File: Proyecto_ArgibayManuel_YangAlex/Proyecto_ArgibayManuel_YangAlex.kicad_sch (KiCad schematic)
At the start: 27 parts, among them J2 Conn_01x04, J3 Conn_01x06, J4 Conn_01x05, SW1 SW_Push, SW2 SW_Push, SW3 SW_Push, SW4 SW_Push, U1 PIC18F258-I_SO, U2 LT1716IS5TRMPBF, U3 LT1716IS5TRMPBF, U7 HDC2010YPAR, U8 TXS0108EPW, Y1 Crystal

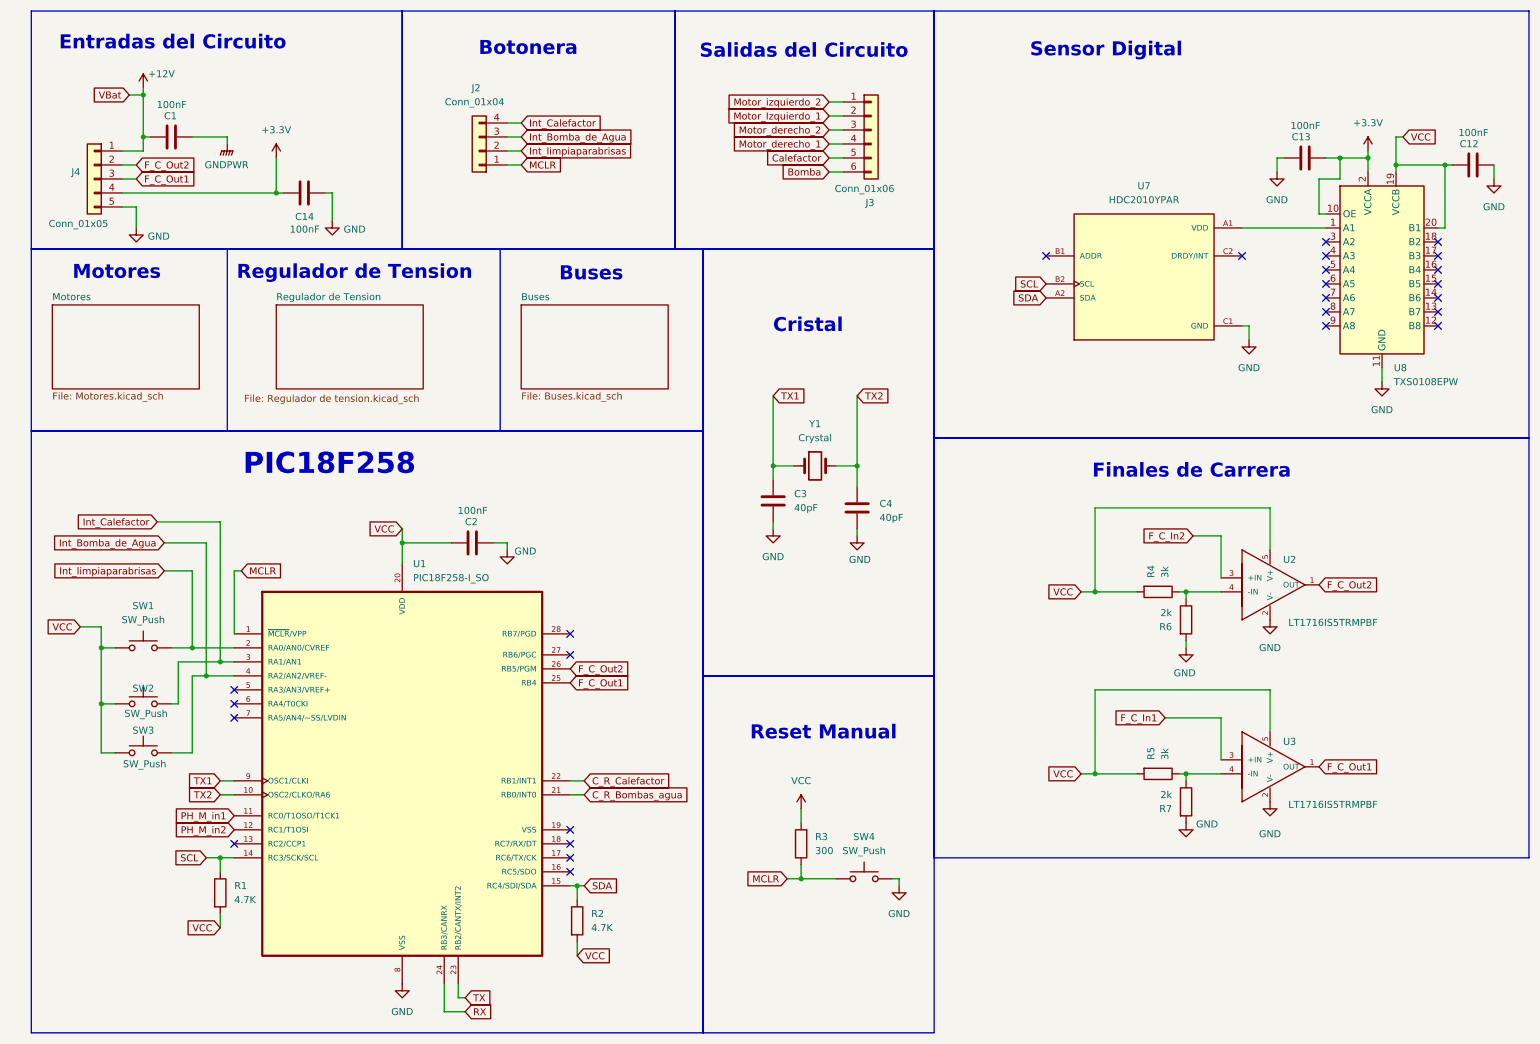
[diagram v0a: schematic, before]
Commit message: icsp
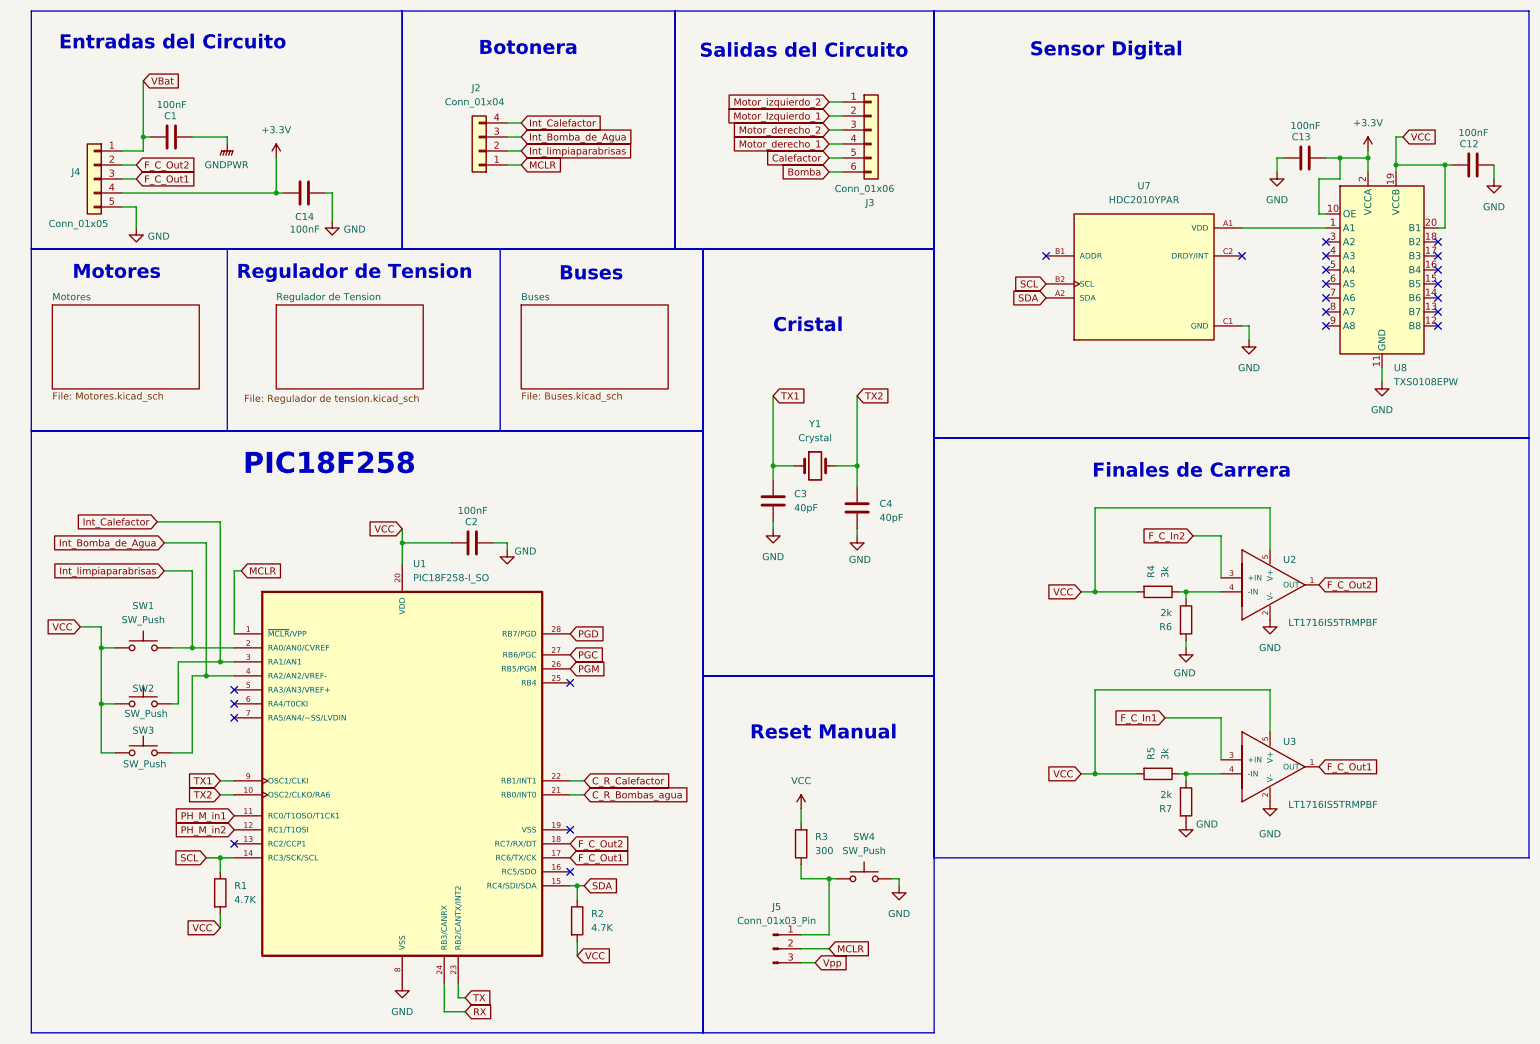
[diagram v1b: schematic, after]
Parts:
- added J5: Conn_01x03_Pin, symbol Connector:Conn_01x03_Pin
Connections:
- net F_C_Out1: now also U1.17 (RC6/TX/CK); no longer U1.25 (RB4)
- net F_C_Out2: now also U1.18 (RC7/RX/DT); no longer U1.26 (RB5/PGM)
- net MCLR: now also J5.2 (Pin_2); no longer R3.1, SW4.1
- net PGC: now reaches U1.27 (RB6/PGC)
- net PGD: now reaches U1.28 (RB7/PGD)
- net +12V renamed VBat
- new net: J5.1 (Pin_1), R3.1, SW4.1
- new net PGM: U1.26 (RB5/PGM)
- new net Vpp: J5.3 (Pin_3)
- no-connect marks 26 -> 23
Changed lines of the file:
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@@
 	)
 	(junction
-		(at 33.02 27.94)
-		(diameter 0)
-		(color 0 0 0 0)
-	)
-	(junction
 		(at 250.19 39.37)
 		(diameter 0)
@@
 	)
 	(junction
-		(at 152.4 170.18)
+		(at 157.48 170.18)
 		(diameter 0)
 		(color 0 0 0 0)
@@
 	)
 	(no_connect
-		(at 110.49 125.73)
-	)
-	(no_connect
 		(at 247.65 59.69)
 	)
@@
 	)
 	(no_connect
-		(at 267.97 57.15)
+		(at 110.49 134.62)
 	)
 	(no_connect
-		(at 110.49 166.37)
+		(at 267.97 57.15)
 	)
 	(no_connect
@@
 	)
 	(no_connect
-		(at 110.49 129.54)
-	)
-	(no_connect
 		(at 267.97 54.61)
 	)
 	(no_connect
-		(at 110.49 163.83)
-	)
-	(no_connect
 		(at 267.97 67.31)
 	)
@@
 	(wire
 		(pts
-			(xy 30.48 27.94) (xy 33.02 27.94)
-		)
-		(stroke
-			(width 0)
-			(type default)
-		)
-	)
-	(wire
-		(pts
 			(xy 205.74 151.13) (xy 213.36 151.13)
 		)
@@
 	(wire
 		(pts
-			(xy 152.4 170.18) (xy 158.75 170.18)
+			(xy 152.4 170.18) (xy 157.48 170.18)
 		)
 		(stroke
@@
 	(wire
 		(pts
-			(xy 66.04 45.72) (xy 67.31 45.72)
+			(xy 157.48 170.18) (xy 157.48 180.34)
 		)
 		(stroke
@@
 	(wire
 		(pts
-			(xy 99.06 109.22) (xy 99.06 110.49)
+			(xy 66.04 45.72) (xy 67.31 45.72)
 		)
 		(stroke
@@
 	(wire
 		(pts
-			(xy 149.86 170.18) (xy 152.4 170.18)
+			(xy 99.06 109.22) (xy 99.06 110.49)
 		)
 		(stroke
@@
 	(wire
 		(pts
-			(xy 33.02 27.94) (xy 33.02 35.56)
-		)
-		(stroke
-			(width 0)
-			(type default)
-		)
-	)
-	(wire
-		(pts
 			(xy 250.19 39.37) (xy 250.19 43.18)
 		)
@@
 	(wire
 		(pts
-			(xy 33.02 26.67) (xy 33.02 27.94)
+			(xy 33.02 25.4) (xy 33.02 35.56)
 		)
 		(stroke
@@
 	(wire
 		(pts
+			(xy 157.48 180.34) (xy 152.4 180.34)
+		)
+		(stroke
+			(width 0)
+			(type default)
+		)
+	)
+	(wire
+		(pts
 			(xy 87.63 194.31) (xy 91.44 194.31)
 		)
@@
 	(wire
 		(pts
+			(xy 157.48 170.18) (xy 158.75 170.18)
+		)
+		(stroke
+			(width 0)
+			(type default)
+		)
+	)
+	(wire
+		(pts
 			(xy 238.76 39.37) (xy 240.03 39.37)
 		)
@@
 	(wire
 		(pts
+			(xy 152.4 182.88) (xy 157.48 182.88)
+		)
+		(stroke
+			(width 0)
+			(type default)
+		)
+	)
+	(wire
+		(pts
 			(xy 25.4 128.27) (xy 27.94 128.27)
 		)
@@
 	(wire
 		(pts
+			(xy 152.4 185.42) (xy 154.94 185.42)
+		)
+		(stroke
+			(width 0)
+			(type default)
+		)
+	)
+	(wire
+		(pts
 			(xy 48.26 35.56) (xy 41.91 35.56)
 		)
@@
 	(global_label "VBat"
 		(shape input)
-		(at 30.48 27.94 180)
+		(at 33.02 25.4 0)
 		(fields_autoplaced yes)
 		(effects
@@
 				(size 1.27 1.27)
 			)
-			(justify right)
+			(justify left)
 		)
 		(property "Intersheetrefs" "${INTERSHEET_REFS}"
-			(at 23.2615 27.94 0)
+			(at 40.2385 25.4 0)
 			(effects
 				(font
 					(size 1.27 1.27)
 				)
-				(justify right)
+				(justify left)
 				(hide yes)
 			)
@@
 	(global_label "F_C_Out2"
 		(shape input)
-		(at 110.49 132.08 0)
+		(at 110.49 163.83 0)
 		(fields_autoplaced yes)
 		(effects
@@
 		)
 		(property "Intersheetrefs" "${INTERSHEET_REFS}"
-			(at 122.1837 132.08 0)
+			(at 122.1837 163.83 0)
 			(effects
 				(font
@@
 	(global_label "MCLR"
 		(shape input)
-		(at 149.86 170.18 180)
+		(at 157.48 182.88 0)
 		(fields_autoplaced yes)
 		(effects
@@
 				(size 1.27 1.27)
 			)
-			(justify right)
+			(justify left)
 		)
 		(property "Intersheetrefs" "${INTERSHEET_REFS}"
-			(at 141.8553 170.18 0)
+			(at 165.4847 182.88 0)
 			(effects
 				(font
 					(size 1.27 1.27)
 				)
-				(justify right)
+				(justify left)
 				(hide yes)
 			)
@@
 		)
 	)
+	(global_label "PGM"
+		(shape input)
+		(at 110.49 132.08 0)
+		(fields_autoplaced yes)
+		(effects
+			(font
+				(size 1.27 1.27)
+			)
+			(justify left)
+		)
+		(property "Intersheetrefs" "${INTERSHEET_REFS}"
+			(at 117.4666 132.08 0)
+			(effects
+				(font
+					(size 1.27 1.27)
+				)
+				(justify left)
+				(hide yes)
+			)
+		)
+	)
 	(global_label "F_C_Out1"
 		(shape input)
-		(at 110.49 134.62 0)
+		(at 110.49 166.37 0)
 		(fields_autoplaced yes)
 		(effects
@@
 		)
 		(property "Intersheetrefs" "${INTERSHEET_REFS}"
-			(at 122.1837 134.62 0)
+			(at 122.1837 166.37 0)
 			(effects
 				(font
@@
 		)
 	)
+	(global_label "Vpp"
+		(shape input)
+		(at 154.94 185.42 0)
+		(fields_autoplaced yes)
+		(effects
+			(font
+				(size 1.27 1.27)
+			)
+			(justify left)
+		)
+		(property "Intersheetrefs" "${INTERSHEET_REFS}"
+			(at 161.3118 185.42 0)
+			(effects
+				(font
+					(size 1.27 1.27)
+				)
+				(justify left)
+				(hide yes)
+			)
+		)
+	)
+	(global_label "PGC"
+		(shape input)
+		(at 110.49 129.54 0)
+		(fields_autoplaced yes)
+		(effects
+			(font
+				(size 1.27 1.27)
+			)
+			(justify left)
+		)
+		(property "Intersheetrefs" "${INTERSHEET_REFS}"
+			(at 117.2852 129.54 0)
+			(effects
+				(font
+					(size 1.27 1.27)
+				)
+				(justify left)
+				(hide yes)
+			)
+		)
+	)
 	(global_label "C_R_Calefactor"
 		(shape input)
@@
 		)
 	)
+	(global_label "PGD"
+		(shape input)
+		(at 110.49 125.73 0)
+		(fields_autoplaced yes)
+		(effects
+			(font
+				(size 1.27 1.27)
+			)
+			(justify left)
+		)
+		(property "Intersheetrefs" "${INTERSHEET_REFS}"
+			(at 117.2852 125.73 0)
+			(effects
+				(font
+					(size 1.27 1.27)
+				)
+				(justify left)
+				(hide yes)
+			)
+		)
+	)
 	(global_label "TX1"
 		(shape input)
@@
 	)
 	(symbol
+		(lib_id "Connector:Conn_01x03_Pin")
+		(at 147.32 182.88 0)
+		(unit 1)
+		(exclude_from_sim no)
+		(in_bom yes)
+		(on_board yes)
+		(dnp no)
+		(fields_autoplaced yes)
+		(property "Reference" "J5"
+			(at 147.955 175.26 0)
+			(effects
+				(font
+					(size 1.27 1.27)
+				)
+			)
+		)
+		(property "Value" "Conn_01x03_Pin"
+			(at 147.955 177.8 0)
+			(effects
+				(font
+					(size 1.27 1.27)
+				)
+			)
+		)
+		(property "Footprint" ""
+			(at 147.32 182.88 0)
+			(effects
+				(font
+					(size 1.27 1.27)
+				)
+				(hide yes)
+			)
+		)
+		(property "Datasheet" "~"
+			(at 147.32 182.88 0)
+			(effects
+				(font
+					(size 1.27 1.27)
+				)
+				(hide yes)
+			)
+		)
+		(property "Description" "Generic connector, single row, 01x03, script generated"
+			(at 147.32 182.88 0)
+			(effects
+				(font
+					(size 1.27 1.27)
+				)
+				(hide yes)
+			)
+		)
+		(pin "3"
+		)
+		(pin "1"
+		)
+		(pin "2"
+		)
+		(instances
+			(project ""
+				(path "/b2dde924-33f5-41ab-a1bf-811873450a89"
+					(reference "J5")
+					(unit 1)
+				)
+			)
+		)
+	)
+	(symbol
 		(lib_id "Device:R")
 		(at 217.17 151.13 270)
@@
 					(unit 1)
 				)
-			)
-		)
-	)
-	(symbol
-		(lib_id "power:+12V")
-		(at 33.02 26.67 0)
-		(unit 1)
-		(exclude_from_sim no)
-		(in_bom yes)
-		(on_board yes)
-		(dnp no)
-		(property "Reference" "#PWR02"
-			(at 33.02 30.48 0)
-			(effects
-				(font
-					(size 1.27 1.27)
-				)
-				(hide yes)
-			)
-		)
-		(property "Value" "+12V"
-			(at 36.322 24.13 0)
-			(effects
-				(font
-					(size 1.27 1.27)
-				)
-			)
-		)
-		(property "Footprint" ""
-			(at 33.02 26.67 0)
-			(effects
-				(font
-					(size 1.27 1.27)
-				)
-				(hide yes)
-			)
-		)
-		(property "Datasheet" ""
-			(at 33.02 26.67 0)
-			(effects
-				(font
-					(size 1.27 1.27)
-				)
-				(hide yes)
-			)
-		)
-		(property "Description" "Power symbol creates a global label with name \"+12V\""
-			(at 33.02 26.67 0)
-			(effects
-				(font
-					(size 1.27 1.27)
-				)
-				(hide yes)
-			)
-		)
-		(pin "1"
-		)
-		(instances
-			(project ""
-				(path "/b2dde924-33f5-41ab-a1bf-811873450a89"
-					(reference "#PWR02")
-					(unit 1)
-				)
